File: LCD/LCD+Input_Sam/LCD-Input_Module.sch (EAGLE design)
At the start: 23 parts

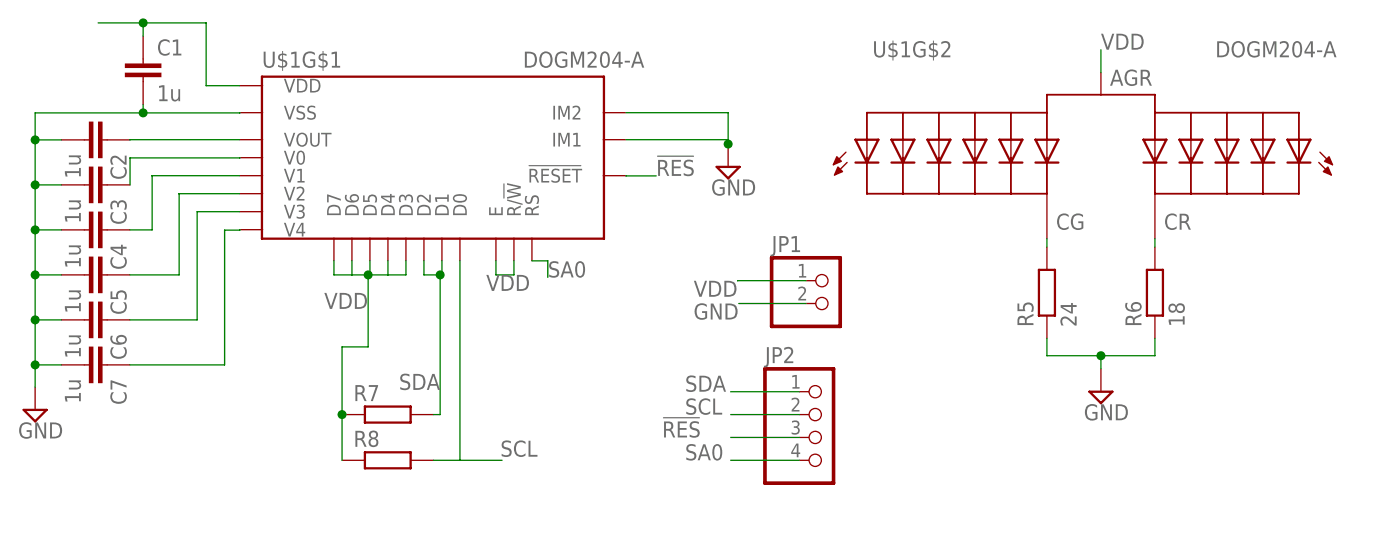
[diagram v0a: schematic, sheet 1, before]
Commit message: LCD PCB finished (again)
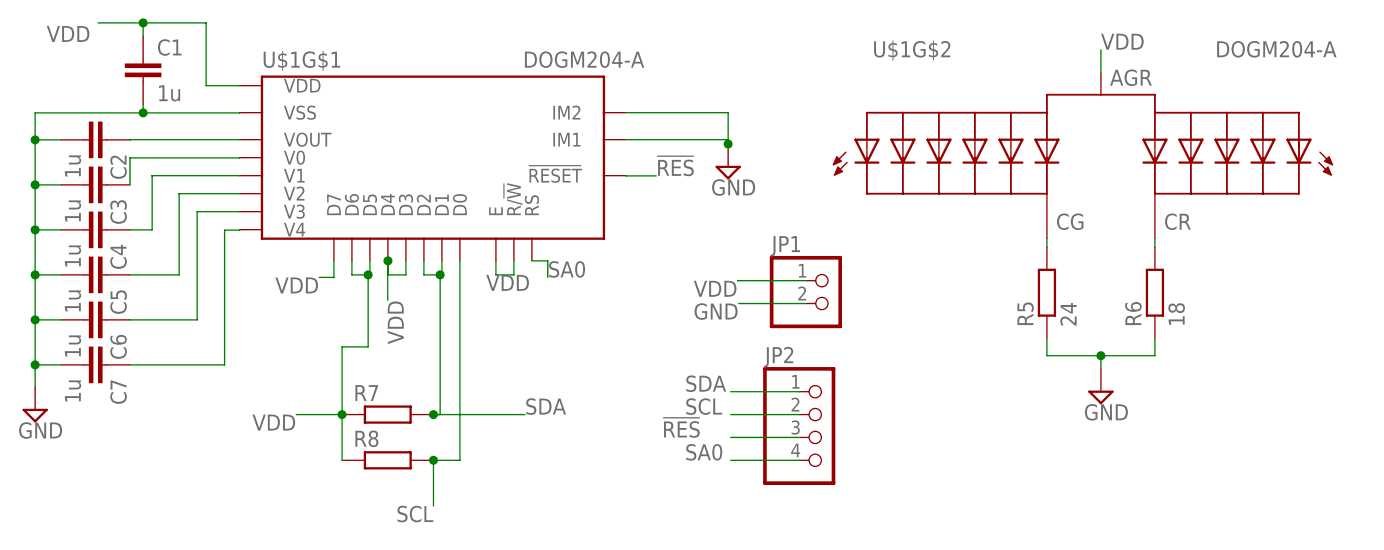
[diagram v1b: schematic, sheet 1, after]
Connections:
- removed net N$10: C1.1, U$1G$1.VDD
- net VDD: now also C1.1, U$1G$1.VDD
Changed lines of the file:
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@@
 <wire x1="49.2" y1="46" x2="49.2" y2="47.565" width="0.1524" layer="91"/>
 <junction x="49" y="46"/>
-<label x="49" y="35" size="1.778" layer="95" rot="R180"/>
 <pinref part="R7" gate="G$1" pin="2"/>
 <wire x1="49" y1="46" x2="49" y2="30.48" width="0.1524" layer="91"/>
 <wire x1="49" y1="30.48" x2="48.26" y2="30.48" width="0.1524" layer="91"/>
+<label x="58.42" y="30.48" size="1.778" layer="95"/>
+<wire x1="58.42" y1="30.48" x2="48.26" y2="30.48" width="0.1524" layer="91"/>
+<junction x="48.26" y="30.48"/>
 </segment>
 <segment>
@@
 </segment>
 <segment>
-<pinref part="U$1" gate="G$1" pin="D7"/>
-<wire x1="37.2" y1="47.565" x2="37.2" y2="46" width="0.1524" layer="91"/>
-<wire x1="37.2" y1="46" x2="39.2" y2="46" width="0.1524" layer="91"/>
 <pinref part="U$1" gate="G$1" pin="D6"/>
 <wire x1="39.2" y1="46" x2="39.2" y2="47.565" width="0.1524" layer="91"/>
 <pinref part="U$1" gate="G$1" pin="D5"/>
 <wire x1="41.2" y1="47.565" x2="41.2" y2="46" width="0.1524" layer="91"/>
-<pinref part="U$1" gate="G$1" pin="D4"/>
-<wire x1="41.2" y1="46" x2="43.2" y2="46" width="0.1524" layer="91"/>
-<wire x1="43.2" y1="46" x2="43.2" y2="47.565" width="0.1524" layer="91"/>
-<pinref part="U$1" gate="G$1" pin="D3"/>
-<wire x1="45.2" y1="47.565" x2="45.2" y2="46" width="0.1524" layer="91"/>
-<wire x1="45.2" y1="46" x2="43.2" y2="46" width="0.1524" layer="91"/>
 <wire x1="39.2" y1="46" x2="41" y2="46" width="0.1524" layer="91"/>
 <wire x1="41" y1="46" x2="41.2" y2="46" width="0.1524" layer="91"/>
 <junction x="41" y="46"/>
-<label x="41" y="44" size="1.778" layer="95" rot="R180"/>
 <pinref part="R7" gate="G$1" pin="1"/>
 <wire x1="38.1" y1="30.48" x2="38.1" y2="38" width="0.1524" layer="91"/>
@@
 <wire x1="38.1" y1="25.4" x2="38.1" y2="30.48" width="0.1524" layer="91"/>
 <junction x="38.1" y="30.48"/>
-</segment>
-</net>
-<net name="!RES" class="0">
-<segment>
-<pinref part="U$1" gate="G$1" pin="!RESET"/>
-<wire x1="69.66" y1="57.025" x2="69.66" y2="57" width="0.1524" layer="91"/>
-<wire x1="69.66" y1="57" x2="73" y2="57" width="0.1524" layer="91"/>
-<label x="73" y="57" size="1.778" layer="95"/>
-</segment>
-<segment>
-<pinref part="JP2" gate="A" pin="3"/>
-<wire x1="81.28" y1="27.94" x2="88.9" y2="27.94" width="0.1524" layer="91"/>
-<label x="73.66" y="27.94" size="1.778" layer="95"/>
-</segment>
-</net>
-<net name="SCL" class="0">
-<segment>
-<pinref part="R8" gate="G$1" pin="2"/>
-<pinref part="U$1" gate="G$1" pin="D0"/>
-<wire x1="48.26" y1="25.4" x2="51.2" y2="25.4" width="0.1524" layer="91"/>
-<wire x1="51.2" y1="25.4" x2="51.2" y2="47.565" width="0.1524" layer="91"/>
-<label x="55.68" y="25.8" size="1.778" layer="95"/>
-<wire x1="51.2" y1="25.4" x2="55.88" y2="25.4" width="0.1524" layer="91"/>
-</segment>
-<segment>
-<pinref part="JP2" gate="A" pin="2"/>
-<wire x1="81.28" y1="30.48" x2="88.9" y2="30.48" width="0.1524" layer="91"/>
-<label x="76.2" y="30.48" size="1.778" layer="95"/>
-</segment>
-</net>
-<net name="N$11" class="0">
-<segment>
-<pinref part="U$1" gate="G$1" pin="VOUT"/>
-<pinref part="C2" gate="G$1" pin="1"/>
-<wire x1="26.74" y1="61.025" x2="14.54" y2="61.025" width="0.1524" layer="91"/>
-<wire x1="14.54" y1="61.025" x2="14.54" y2="61" width="0.1524" layer="91"/>
-</segment>
-</net>
-<net name="N$9" class="0">
-<segment>
-<pinref part="C7" gate="G$1" pin="1"/>
-<wire x1="14.54" y1="36" x2="25.05" y2="36" width="0.1524" layer="91"/>
-<wire x1="25.05" y1="36" x2="25.05" y2="50.975" width="0.1524" layer="91"/>
-<pinref part="U$1" gate="G$1" pin="V4"/>
-<wire x1="25.05" y1="50.975" x2="26.74" y2="50.975" width="0.1524" layer="91"/>
-<wire x1="26.74" y1="50.975" x2="26.74" y2="51.025" width="0.1524" layer="91"/>
-</segment>
-</net>
-<net name="N$15" class="0">
-<segment>
-<pinref part="R5" gate="G$1" pin="2"/>
-<pinref part="U$1" gate="G$2" pin="CG"/>
-<wire x1="116.42" y1="49.1" x2="116.42" y2="50.02" width="0.1524" layer="91"/>
-</segment>
-</net>
-<net name="N$19" class="0">
-<segment>
-<pinref part="R6" gate="G$1" pin="2"/>
-<pinref part="U$1" gate="G$2" pin="CR"/>
-<wire x1="128.42" y1="49.1" x2="128.42" y2="50.02" width="0.1524" layer="91"/>
-</segment>
-</net>
-<net name="N$10" class="0">
+<wire x1="38.1" y1="30.48" x2="33.02" y2="30.48" width="0.1524" layer="91"/>
+<label x="33.02" y="30.48" size="1.778" layer="95" rot="R180"/>
+</segment>
 <segment>
 <pinref part="C1" gate="G$1" pin="1"/>
@@
 <wire x1="23" y1="74" x2="16" y2="74" width="0.1524" layer="91"/>
 <junction x="16" y="74"/>
-</segment>
-</net>
+<label x="10.16" y="73.66" size="1.778" layer="95" rot="R180"/>
+</segment>
+<segment>
+<pinref part="U$1" gate="G$1" pin="D7"/>
+<wire x1="37.2" y1="47.565" x2="37.2" y2="45.72" width="0.1524" layer="91"/>
+<wire x1="37.2" y1="45.72" x2="35.56" y2="45.72" width="0.1524" layer="91"/>
+<label x="35.56" y="45.72" size="1.778" layer="95" rot="R180"/>
+</segment>
+<segment>
+<pinref part="U$1" gate="G$1" pin="D4"/>
+<wire x1="43.2" y1="46" x2="43.2" y2="47.565" width="0.1524" layer="91"/>
+<pinref part="U$1" gate="G$1" pin="D3"/>
+<wire x1="45.2" y1="47.565" x2="45.2" y2="46" width="0.1524" layer="91"/>
+<wire x1="45.2" y1="46" x2="43.2" y2="46" width="0.1524" layer="91"/>
+<wire x1="43.2" y1="47.565" x2="43.18" y2="47.565" width="0.1524" layer="91"/>
+<wire x1="43.18" y1="47.565" x2="43.18" y2="43.18" width="0.1524" layer="91"/>
+<junction x="43.2" y="47.565"/>
+<label x="43.18" y="43.18" size="1.778" layer="95" rot="R270"/>
+</segment>
+</net>
+<net name="!RES" class="0">
+<segment>
+<pinref part="U$1" gate="G$1" pin="!RESET"/>
+<wire x1="69.66" y1="57.025" x2="69.66" y2="57" width="0.1524" layer="91"/>
+<wire x1="69.66" y1="57" x2="73" y2="57" width="0.1524" layer="91"/>
+<label x="73" y="57" size="1.778" layer="95"/>
+</segment>
+<segment>
+<pinref part="JP2" gate="A" pin="3"/>
+<wire x1="81.28" y1="27.94" x2="88.9" y2="27.94" width="0.1524" layer="91"/>
+<label x="73.66" y="27.94" size="1.778" layer="95"/>
+</segment>
+</net>
+<net name="SCL" class="0">
+<segment>
+<pinref part="JP2" gate="A" pin="2"/>
+<wire x1="81.28" y1="30.48" x2="88.9" y2="30.48" width="0.1524" layer="91"/>
+<label x="76.2" y="30.48" size="1.778" layer="95"/>
+</segment>
+<segment>
+<pinref part="U$1" gate="G$1" pin="D0"/>
+<pinref part="R8" gate="G$1" pin="2"/>
+<wire x1="51.2" y1="47.565" x2="51.2" y2="25.4" width="0.1524" layer="91"/>
+<wire x1="51.2" y1="25.4" x2="48.26" y2="25.4" width="0.1524" layer="91"/>
+<wire x1="48.26" y1="25.4" x2="48.26" y2="20.32" width="0.1524" layer="91"/>
+<junction x="48.26" y="25.4"/>
+<label x="48.26" y="20.32" size="1.778" layer="95" rot="R180"/>
+</segment>
+</net>
+<net name="N$11" class="0">
+<segment>
+<pinref part="U$1" gate="G$1" pin="VOUT"/>
+<pinref part="C2" gate="G$1" pin="1"/>
+<wire x1="26.74" y1="61.025" x2="14.54" y2="61.025" width="0.1524" layer="91"/>
+<wire x1="14.54" y1="61.025" x2="14.54" y2="61" width="0.1524" layer="91"/>
+</segment>
+</net>
+<net name="N$9" class="0">
+<segment>
+<pinref part="C7" gate="G$1" pin="1"/>
+<wire x1="14.54" y1="36" x2="25.05" y2="36" width="0.1524" layer="91"/>
+<wire x1="25.05" y1="36" x2="25.05" y2="50.975" width="0.1524" layer="91"/>
+<pinref part="U$1" gate="G$1" pin="V4"/>
+<wire x1="25.05" y1="50.975" x2="26.74" y2="50.975" width="0.1524" layer="91"/>
+<wire x1="26.74" y1="50.975" x2="26.74" y2="51.025" width="0.1524" layer="91"/>
+</segment>
+</net>
+<net name="N$15" class="0">
+<segment>
+<pinref part="R5" gate="G$1" pin="2"/>
+<pinref part="U$1" gate="G$2" pin="CG"/>
+<wire x1="116.42" y1="49.1" x2="116.42" y2="50.02" width="0.1524" layer="91"/>
+</segment>
+</net>
+<net name="N$19" class="0">
+<segment>
+<pinref part="R6" gate="G$1" pin="2"/>
+<pinref part="U$1" gate="G$2" pin="CR"/>
+<wire x1="128.42" y1="49.1" x2="128.42" y2="50.02" width="0.1524" layer="91"/>
+</segment>
+</net>
